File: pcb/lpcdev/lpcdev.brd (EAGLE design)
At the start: 100 x 80 mm, 83 parts, among them IC1 LPC1517BJD48, IC2 DRV8313, IC3 FT231X, IC4 LP2985-3V3, IC5 DRV8313, IC6 DRV8313, Q1 16MHz

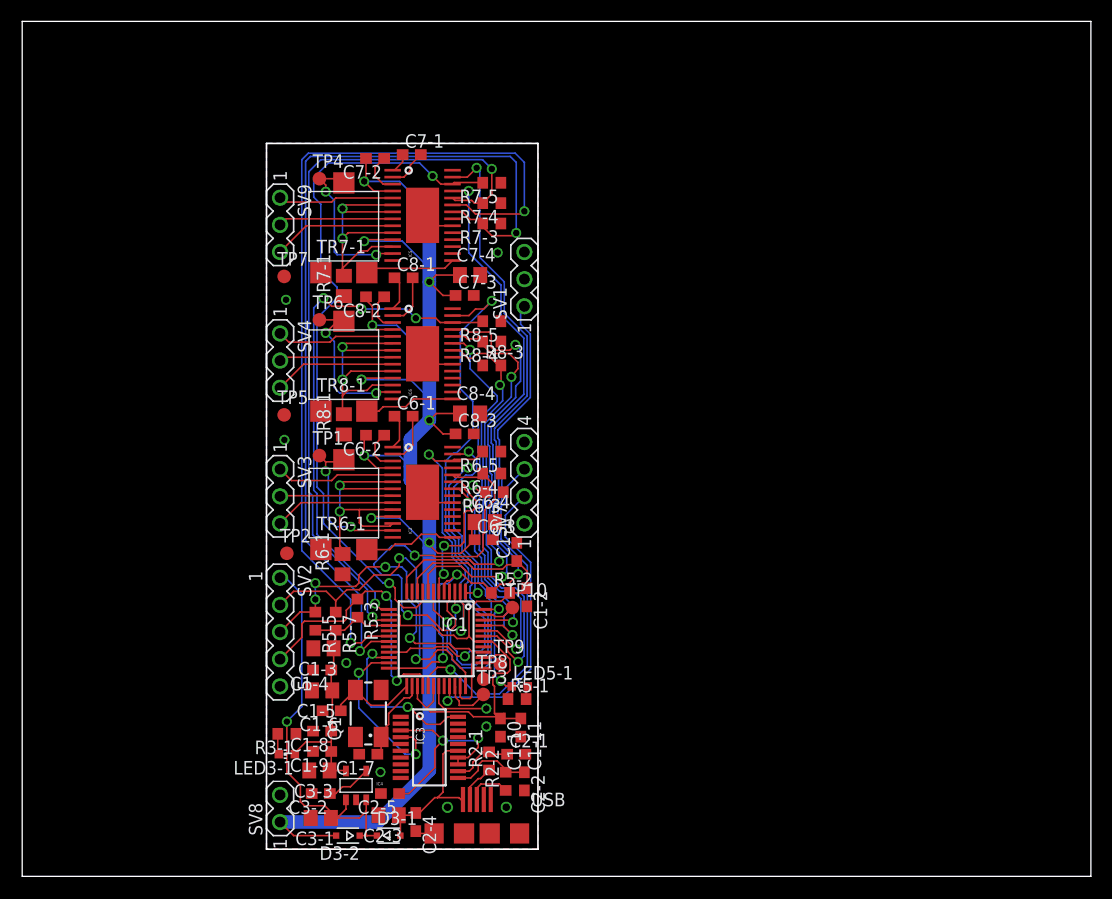
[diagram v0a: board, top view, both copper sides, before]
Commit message: final touchup and gerber generating
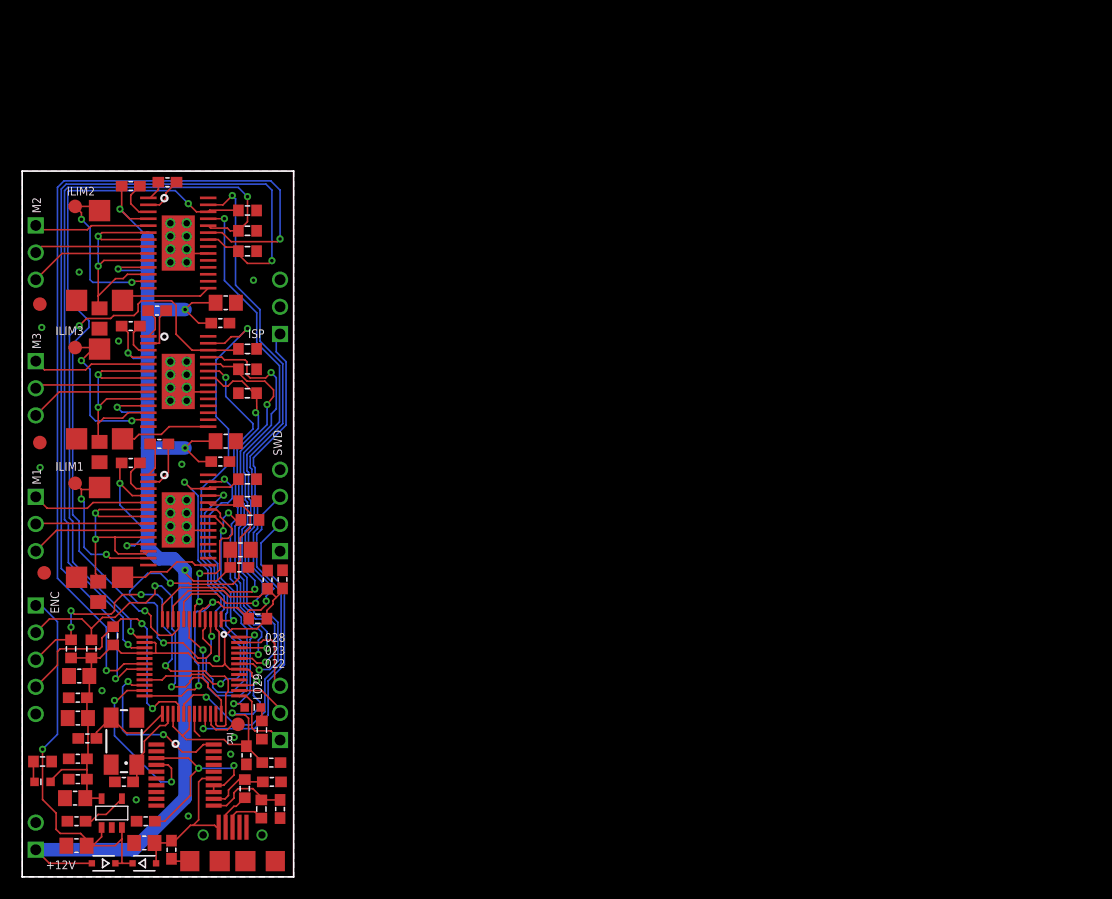
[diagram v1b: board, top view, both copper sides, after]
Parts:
- removed LED5-1: Green, led:CHIP-LED0603
- removed SV1: ISP, lpclib:MA03-1
- removed SV2: ENCODER, lpclib:MA05-1
- removed SV3, SV4, SV9: MOTOR, lpclib:MA03-1
- removed SV7: SWD, lpclib:MA04-1
- removed SV8: +12V, lpclib:MA02-1
- removed TP1, TP10, TP3, TP4, TP6, TP8, TP9: TPB1,27, testpad:B1,27
- added !R, ILIM1, ILIM2, ILIM3: TPB1,27, testpad:B1,27
- added +12V: +12V, lpclib:MA02-1
- added ENC: ENCODER, lpclib:MA05-1
- added GPIO: GPIO, lpclib:MA03-1
- added ISP: ISP, lpclib:MA03-1
- added L029: Green, led:CHIP-LED0603
- added M1, M2, M3: MOTOR, lpclib:MA03-1
- added SWD: SWD, lpclib:MA04-1
- moved R5-1 24.1 mm to (22.4, 13.7), turned to 90 degrees
- moved C1-10 23.9 mm to (21.0, 11.3)
- moved C1-11 23.6 mm to (23.3, 10.6), turned to 0 degrees
- moved C1-1 23.5 mm to (23.0, 27.8)
- moved C8-1 23.3 mm to (12.6, 52.9)
- moved R7-1 23.1 mm to (7.24, 52.2)
- moved C8-2 23.0 mm to (10.2, 51.5)
- moved C2-1 23.0 mm to (23.4, 8.84)
- moved C2-2 23.0 mm to (24.1, 6.30)
- moved C6-2 23.0 mm to (10.2, 38.7)
- moved C7-2 23.0 mm to (10.2, 64.6)
- moved IC2 23.0 mm to (14.6, 33.4)
- moved IC5 23.0 mm to (14.6, 59.3)
- moved IC6 23.0 mm to (14.6, 46.3)
- moved R2-1 23.0 mm to (20.8, 8.20)
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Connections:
- net !RESET: now also !R.TP; no longer TP3.TP
- net +12V: now also +12V.1; no longer SV8.1
- net DRV1_COMPN: now also ILIM1.TP; no longer TP1.TP
- net DRV1_OUT1: now also M1.1; no longer SV3.1
- net DRV1_OUT2: now also M1.2; no longer SV3.2
- net DRV1_OUT3: now also M1.3; no longer SV3.3
- net DRV2_COMPN1: now also ILIM2.TP; no longer TP4.TP
- net DRV2_OUT1: now also M2.1; no longer SV9.1
- net DRV2_OUT2: now also M2.2; no longer SV9.2
- net DRV2_OUT3: now also M2.3; no longer SV9.3
- net DRV3_COMPN2: now also ILIM3.TP; no longer TP6.TP
- net DRV3_OUT1: now also M3.1; no longer SV4.1
- net DRV3_OUT2: now also M3.2; no longer SV4.2
- net DRV3_OUT3: now also M3.3; no longer SV4.3
- net GND: now also +12V.2, ENC.5, ISP.2, SWD.4; no longer SV1.2, SV2.5, SV7.4, SV8.2
- net ISP_01: now also ISP.1; no longer SV1.1
- net LED1: now also L029.C; no longer LED5-1.C
- net PIO0_22: now also GPIO.1; no longer TP8.TP
- net PIO0_23: now also GPIO.2; no longer TP9.TP
- net PIO0_28: now also GPIO.3; no longer TP10.TP
- net PIO0_29: now also L029.A; no longer LED5-1.A
- net QEI_IDX: now also ENC.4; no longer SV2.4
- net QEI_PHA: now also ENC.2; no longer SV2.2
- net QEI_PHB: now also ENC.3; no longer SV2.3
- net REG_VIN: now also ENC.1; no longer SV2.1
- net SWCLK: now also SWD.3; no longer SV7.3
- net SWDIO: now also SWD.2; no longer SV7.2
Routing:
- net +12V: track 157.4 -> 145.9 mm
- net PIO0_22: track 1.07 -> 7.10 mm
- net PIO0_28: track 3.13 -> 7.71 mm
- net DRV3_EN1: track 49.1 -> 53.0 mm, vias 4 -> 2
- net GND: track 18.5 -> 15.1 mm, vias 7 -> 35
- net PIO0_23: track 1.64 -> 4.92 mm
- net DRV3_IN2: track 46.1 -> 42.8 mm
- net DRV3_IN3: track 35.9 -> 33.5 mm
- net DRV3_EN2: track 42.0 -> 39.6 mm
- net PIO0_29: track 9.89 -> 10.8 mm
- net !RESET: track 4.66 -> 3.97 mm
- net DRV2_EN1: track 66.1 -> 66.7 mm
- net DRV3_CPH2: track 4.92 -> 4.36 mm
- net DRV3_EN3: track 36.0 -> 35.5 mm
- net +3V3: track 89.2 -> 89.3 mm, vias 0 -> 2
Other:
- board size 100 x 80 mm -> 25.4 x 66 mm
- board text added: "028 023 022"
- board text added: "Gimbal controller - rev1"
- board text added: "dlofstrom"
